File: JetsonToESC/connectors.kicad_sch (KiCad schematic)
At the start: 12 parts, among them J1 Conn_01x12, J2 Conn_01x03, J3 Conn_01x02, J4 Screw_Terminal_01x01, J5 Screw_Terminal_01x01

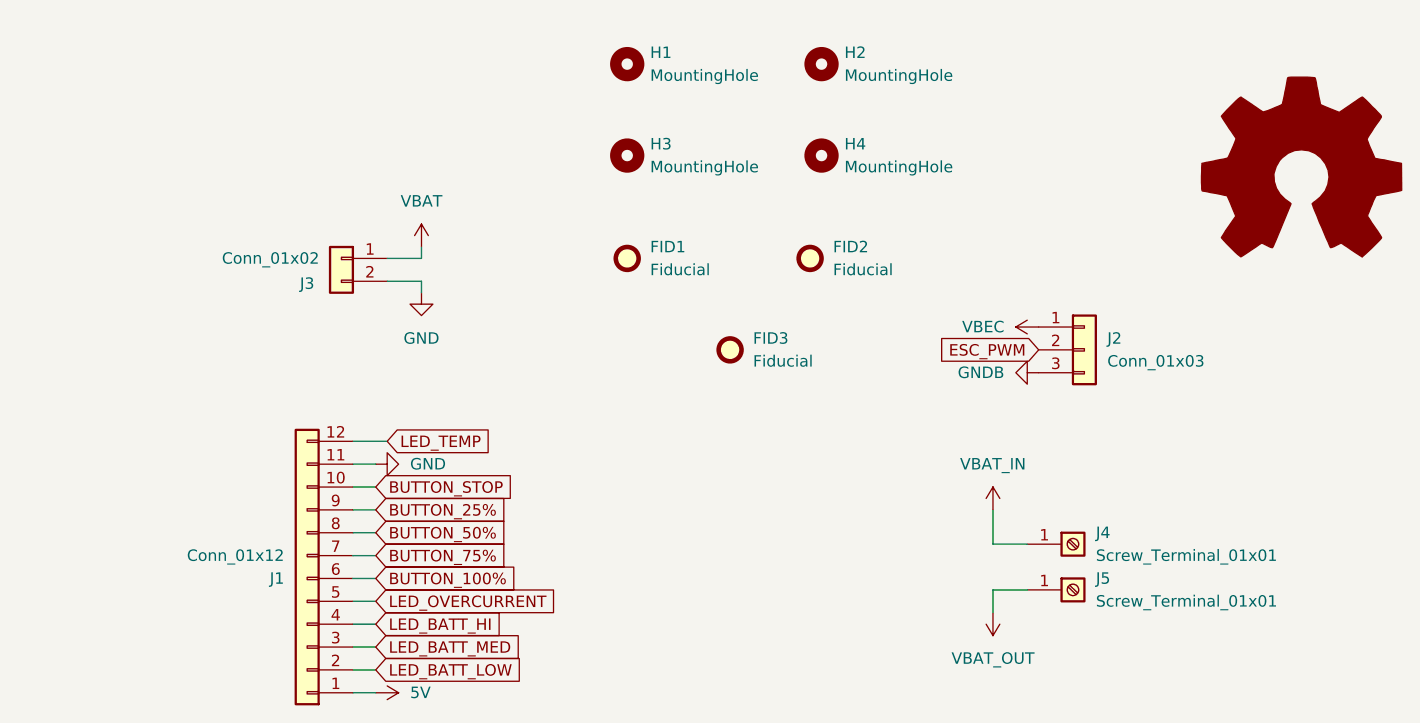
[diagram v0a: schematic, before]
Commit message: Design and routing done
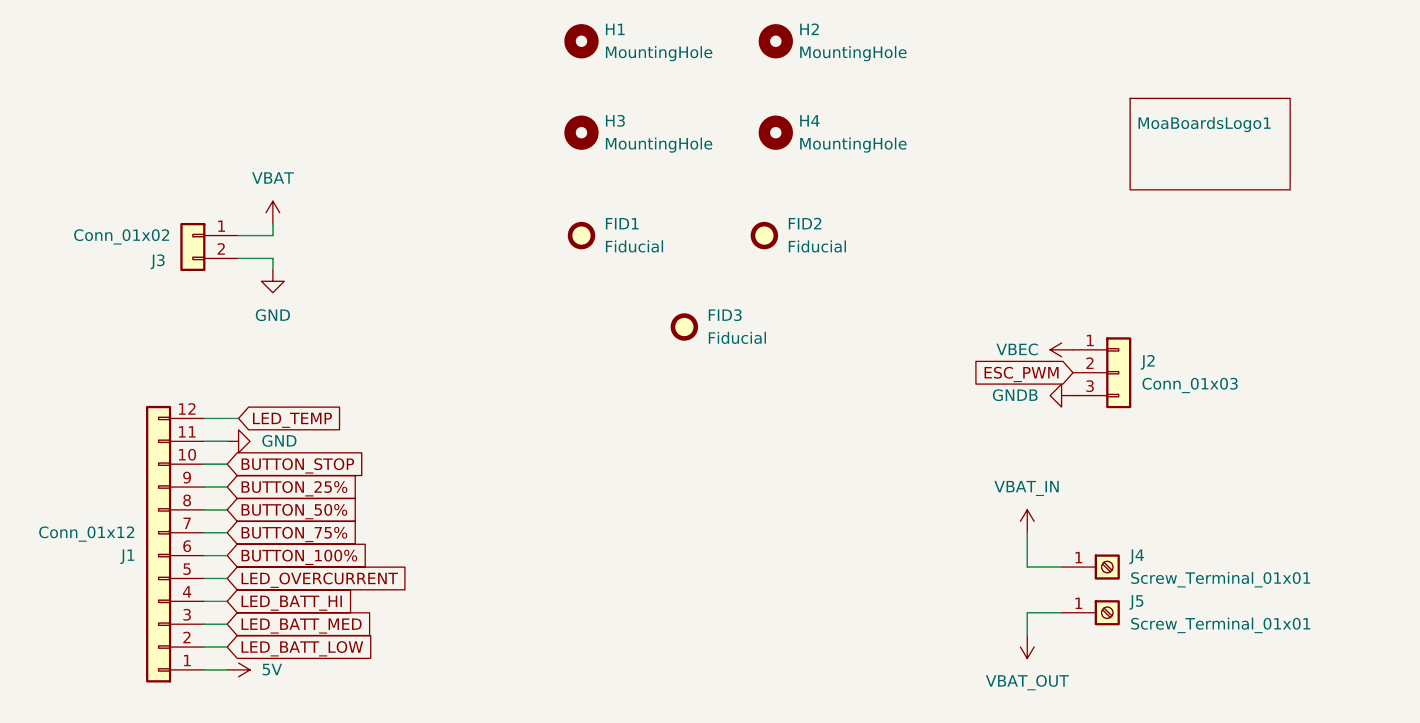
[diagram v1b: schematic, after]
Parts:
- added MoaBoardsLogo1: ~, Logos:MoaBoards, symbol Logos:LogoMoaBoards
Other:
- moved on the sheet: FID1, FID2, FID3, H1, H2, H3, H4, J1, J2, J3, J4, J5
